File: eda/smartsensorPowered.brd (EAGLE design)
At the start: 47 x 26.7 mm, 35 parts, among them Q1 IRFML8244, Q2 IRFML8244, Q3 IRFML8244, Q4 IRFML8244, U1 ISL83491SOIC, U2 ATTINY1634

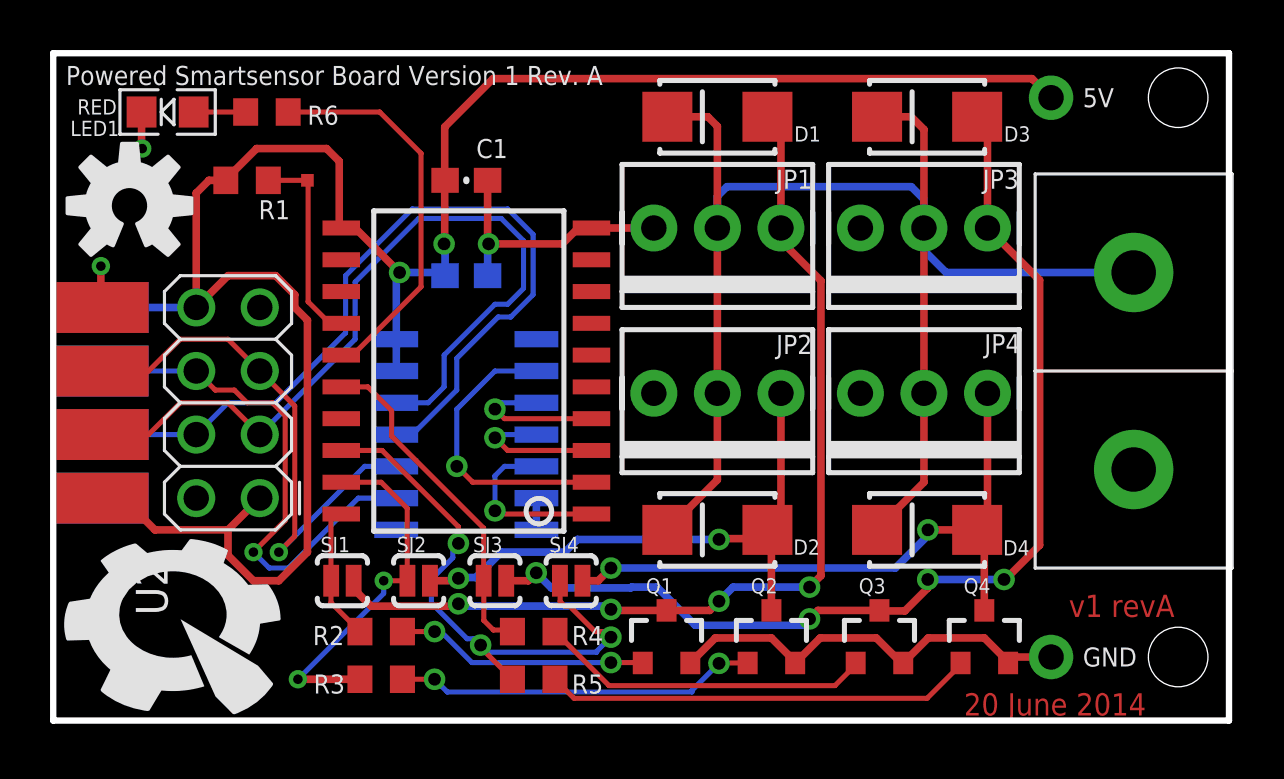
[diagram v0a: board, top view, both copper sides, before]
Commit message: Fixed version of Krystyn ribboncable change
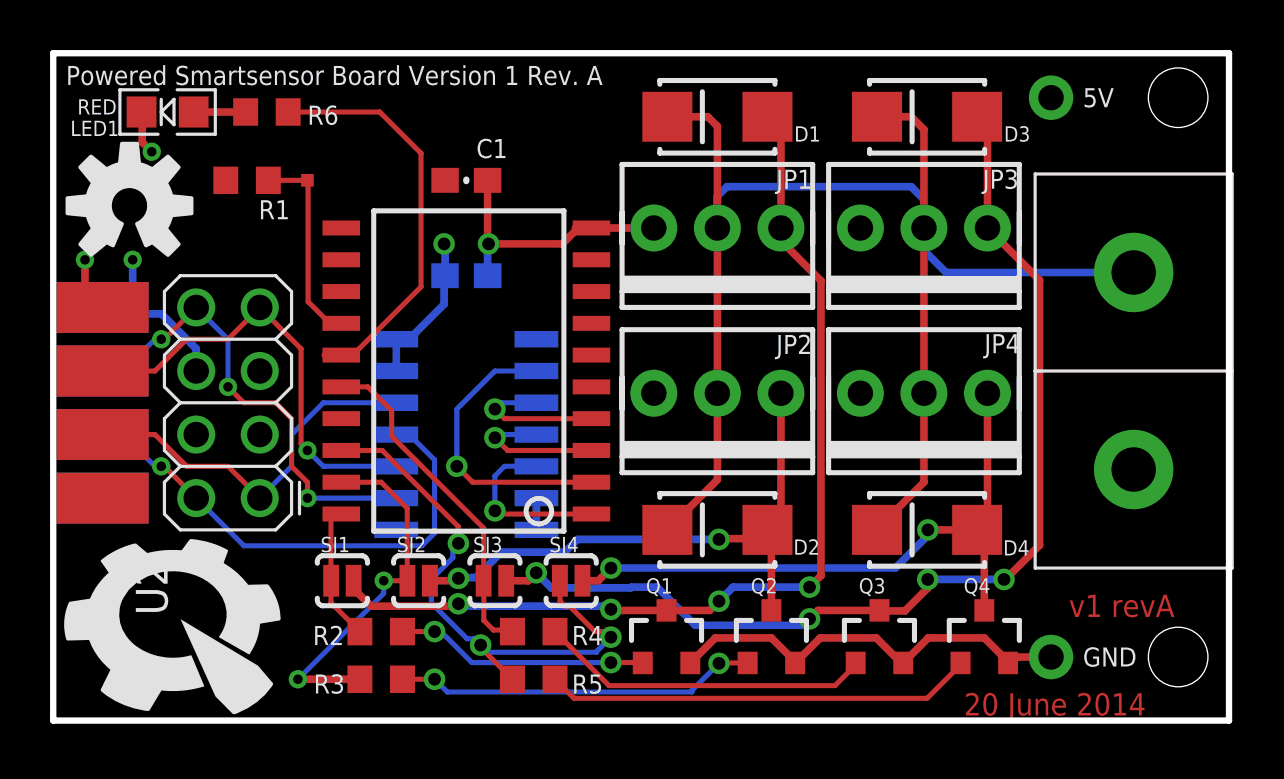
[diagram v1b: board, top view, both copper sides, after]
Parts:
- renumbered U$7 to U$12, U$8 to U$13
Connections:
- net 5V: now also U$12.3, U$12.6; no longer U$12.1, U$12.8
- net A_N: now also U$12.2; no longer U$12.4
- net A_P: now also U$12.1; no longer U$12.3
- net B_N: now also U$12.7; no longer U$12.5
- net B_P: now also U$12.8; no longer U$12.6
- net GND: now also U$12.4, U$12.5; no longer U$12.2, U$12.7
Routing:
- net 5V: track 86.2 -> 14.2 mm
- net A_P: track 32.9 -> 15.5 mm
- net A_N: track 33.7 -> 20.5 mm, vias 0 -> 1
- net B_N: track 21.6 -> 17.7 mm
- net B_P: track 21.2 -> 18.7 mm, vias 1 -> 3
- net TXE: track 5.96 -> 5.32 mm
- net TX: track 7.12 -> 6.49 mm
- net RX: track 11.7 -> 11.1 mm
- net !RXE: track 5.88 -> 5.25 mm
- net LED: track 15.6 -> 16.3 mm
- net IO3: track 13.8 -> 14.4 mm
- net IO4: track 23.4 -> 24.0 mm
- net IO2: track 14.7 -> 15.4 mm
- added copper zone on layer 1, net 5V
